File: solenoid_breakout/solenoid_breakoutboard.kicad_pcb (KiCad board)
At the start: 2 copper layers, 33.5 x 18.5 mm, 9 parts, among them J1 Conn_01x04_Pin, J2 Conn_01x04_Pin, J3 Conn_01x04_Pin, J4 Conn_01x04_Pin, J7 Conn_01x05, J8 Conn_01x05, U1 PCA9536DP

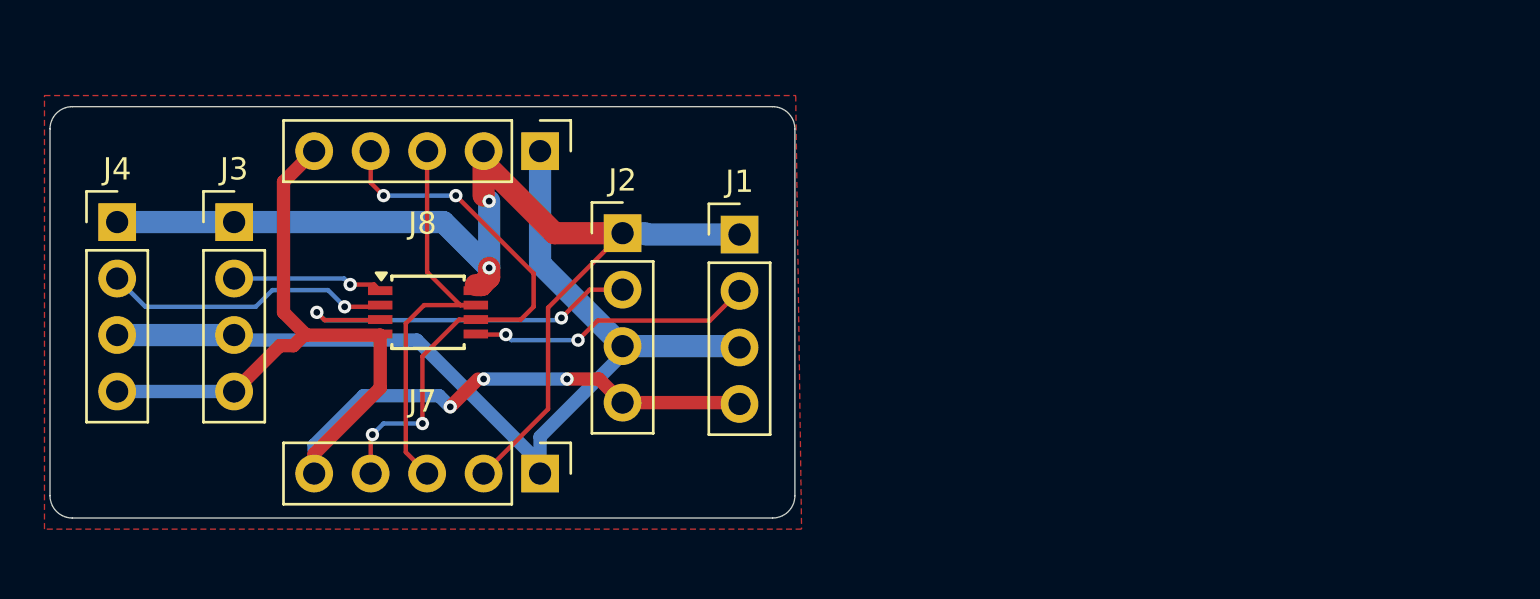
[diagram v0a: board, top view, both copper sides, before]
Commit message: gpio board iteration 2 updated
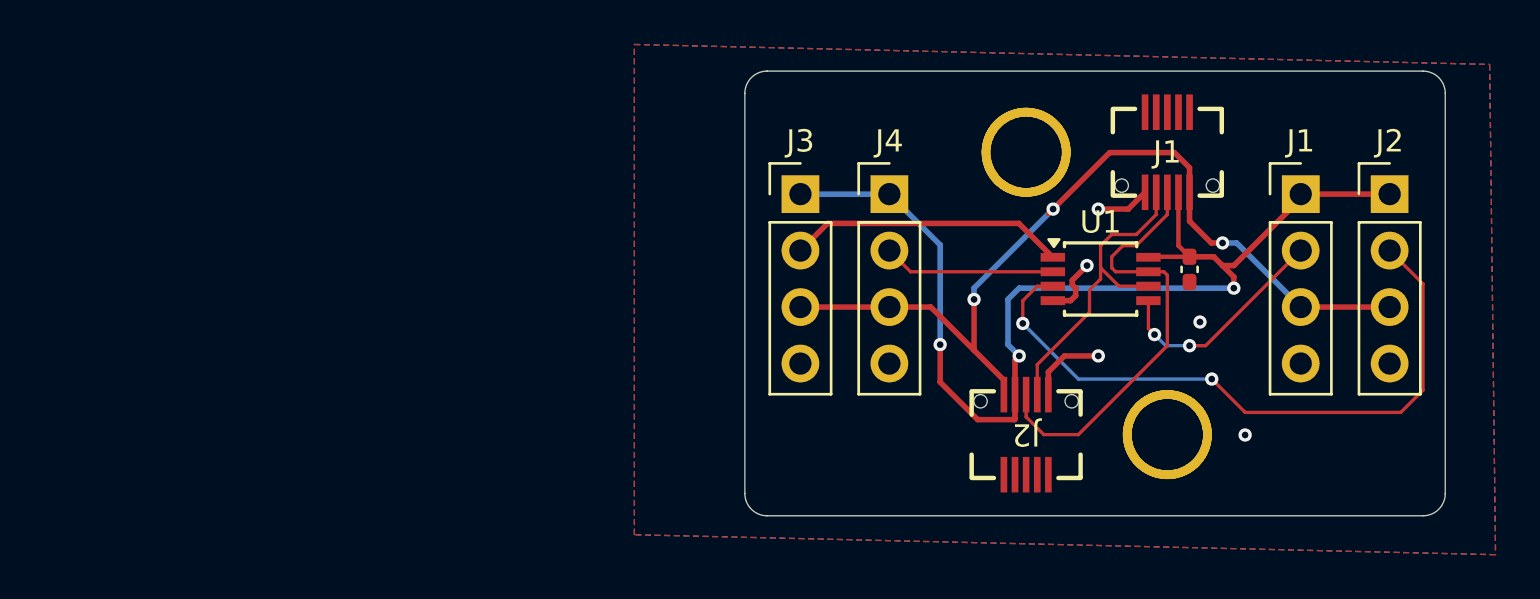
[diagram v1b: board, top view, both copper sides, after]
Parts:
- removed the J1 at (104.3, 55.5)
- removed the J2 at (99.0, 55.4)
- removed J7, J8: Conn_01x05, Connector_PinHeader_2.54mm:PinHeader_1x05_P2.54mm_Vertical
- added ? (x2): , , F.Cu at (123.5, 64.5)
- added ? (x2): , , F.Cu at (117.2, 51.8)
- added C1: 0.1uF, Capacitor_SMD:C_0402_1005Metric_Pad0.74x0.62mm_HandSolder, F.Cu at (124.5, 57.1)
- added J1: Conn_01x04_Pin, Connector_PinHeader_2.54mm:PinHeader_1x04_P2.54mm_Vertical, F.Cu at (129.5, 53.7)
- added J1: Conn_01x10, pcb_footprints:GT-B0502MSV27-10S1101, F.Cu at (123.5, 51.8)
- added J2: Conn_01x10, pcb_footprints:GT-B0502MSV27-10S1101, F.Cu at (117.2, 64.5)
- added J2: Conn_01x04_Pin, Connector_PinHeader_2.54mm:PinHeader_1x04_P2.54mm_Vertical, F.Cu at (133.5, 53.7)
- moved J4 34.8 mm to (111.0, 53.7)
- moved G*** 32.1 mm to (134.0, 54.4)
- moved G*** 31.6 mm to (110.0, 53.9)
- moved U1 30.3 mm to (120.5, 57.5)
- moved J3 25.5 mm to (107.0, 53.7)
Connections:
- U1 pad 6: scl -> /scl
- U1 pad 7: sda -> /sda
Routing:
- net GND: track 52.2 -> 8.79 mm, vias 3 -> 5
- net scl: track 25.1 -> 0.00 mm, vias 4 -> 0
- net /sda: track 0.00 -> 19.9 mm
- net sda: track 18.9 -> 0.00 mm
- net /scl: track 0.00 -> 14.5 mm
- net Net-(J2-Pin_2): track 17.5 -> 29.6 mm
- net Net-(J3-Pin_2): track 6.87 -> 12.5 mm, vias 1 -> 0
- net Net-(J4-Pin_2): track 13.0 -> 7.74 mm, vias 1 -> 0
- net +5V: track 45.1 -> 40.0 mm, vias 0 -> 3
- net Net-(J1-Pin_2): track 12.9 -> 10.2 mm
- net +3.3V: track 51.1 -> 50.4 mm, vias 2 -> 3
- added copper zone on B.Cu, net GND
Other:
- board size 33.5 x 18.5 mm -> 31.5 x 20 mm
- board text added: "Designed by Lakshay Yadav Trung Le"
- board text removed: "Designed by Lakshay Yadav"
